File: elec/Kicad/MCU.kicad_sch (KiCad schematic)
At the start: 7 parts, among them U1 STM32L053C8T6

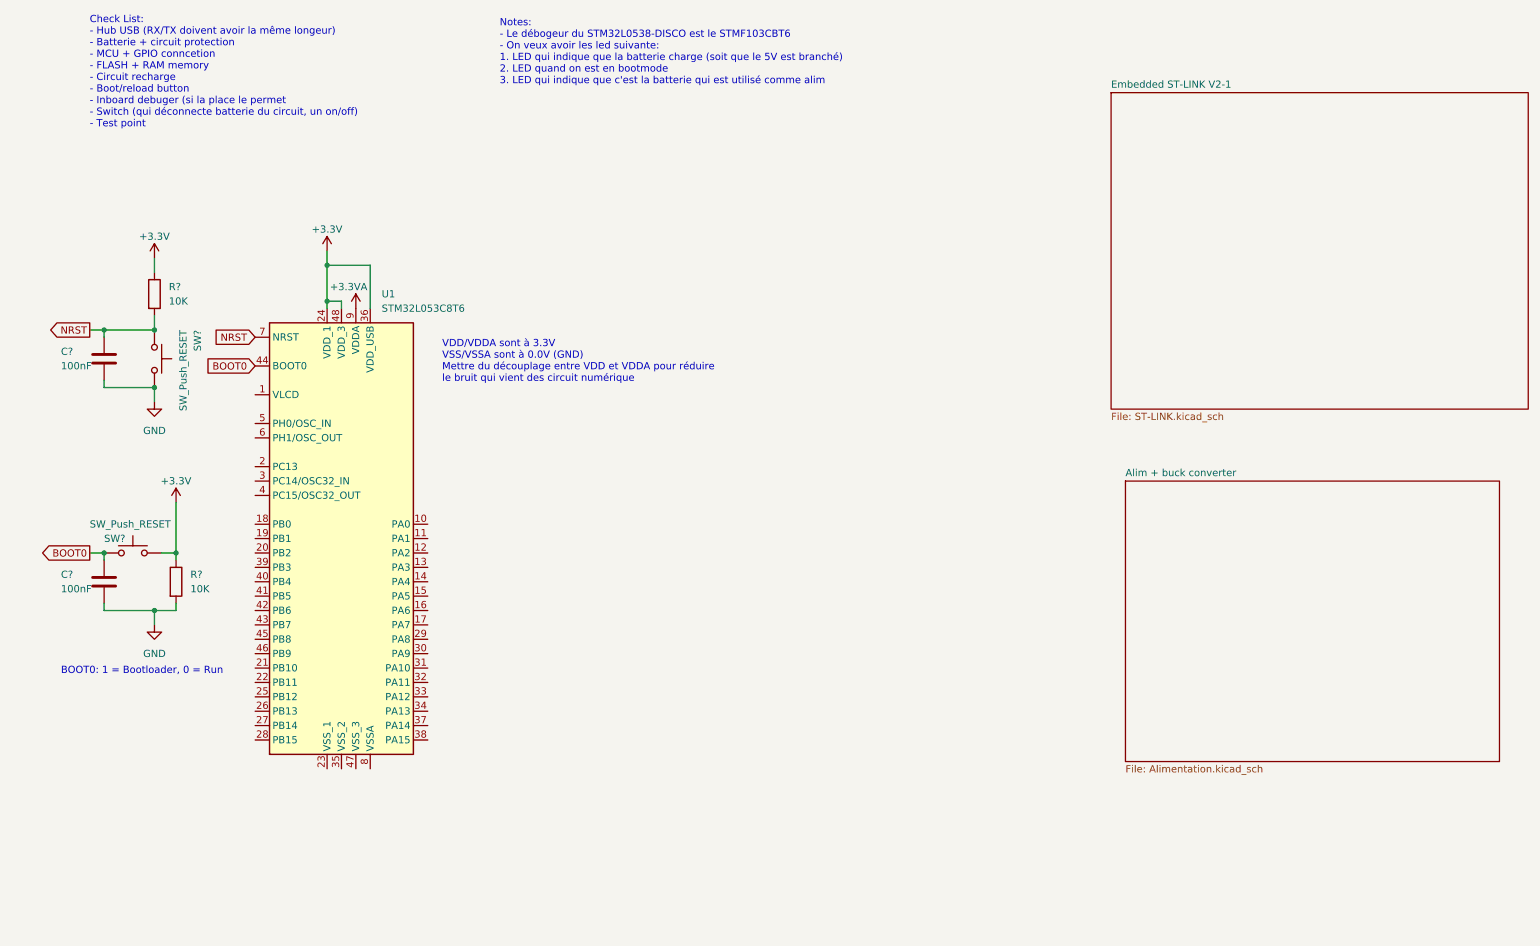
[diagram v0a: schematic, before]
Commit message: merci Linux
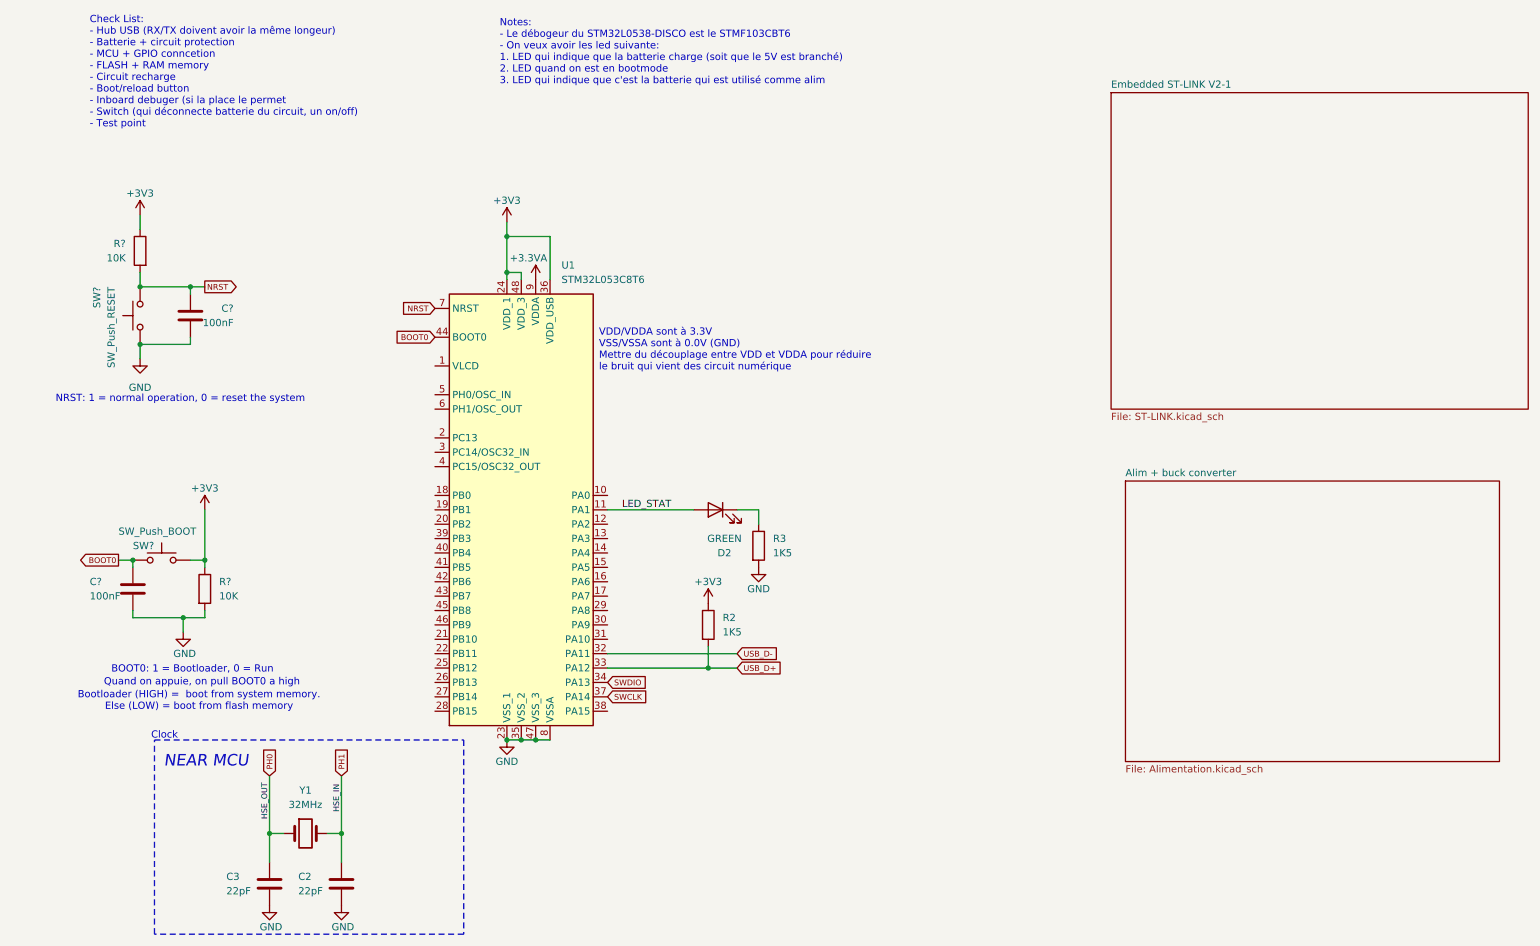
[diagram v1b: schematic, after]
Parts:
- added C2, C3: 22pF, symbol Device:C
- added D2: GREEN, symbol Device:LED
- added R2, R3: 1K5, symbol Device:R
- added Y1: 32MHz, symbol Device:Crystal
- SW?: value SW_Push_RESET -> SW_Push_BOOT
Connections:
- net +3V3: now also R2.1
- net GND: now also U1.23 (VSS_1), U1.35 (VSS_2), U1.47 (VSS_3), U1.8 (VSSA), C2.2, C3.2, R3.2
- net LED_STAT: now reaches U1.11 (PA1)
- net LED_STAT: now also D2.2 (A)
- net USB_D-: now reaches U1.32 (PA11)
- net USB_D+: now reaches U1.33 (PA12)
- net USB_D+: now also R2.2
- net SWDIO: now reaches U1.34 (PA13)
- net SWCLK: now reaches U1.37 (PA14)
- new net: D2.1 (K), R3.1
- new net PH0: C3.1, Y1.1
- new net PH1: C2.1, Y1.2
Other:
- note added: "Bootloader (HIGH) = boot from system memory. Else (LOW) = boot from flash memory"
- note added: "Clock"
- note added: "NEAR MCU"
- note added: "NRST: 1 = normal operation, 0 = reset the system"
- note added: "Quand on appuie, on pull BOOT0 a high"
- moved on the sheet: C?, R?, SW?, U1
